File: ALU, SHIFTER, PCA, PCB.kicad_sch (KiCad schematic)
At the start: 14 parts

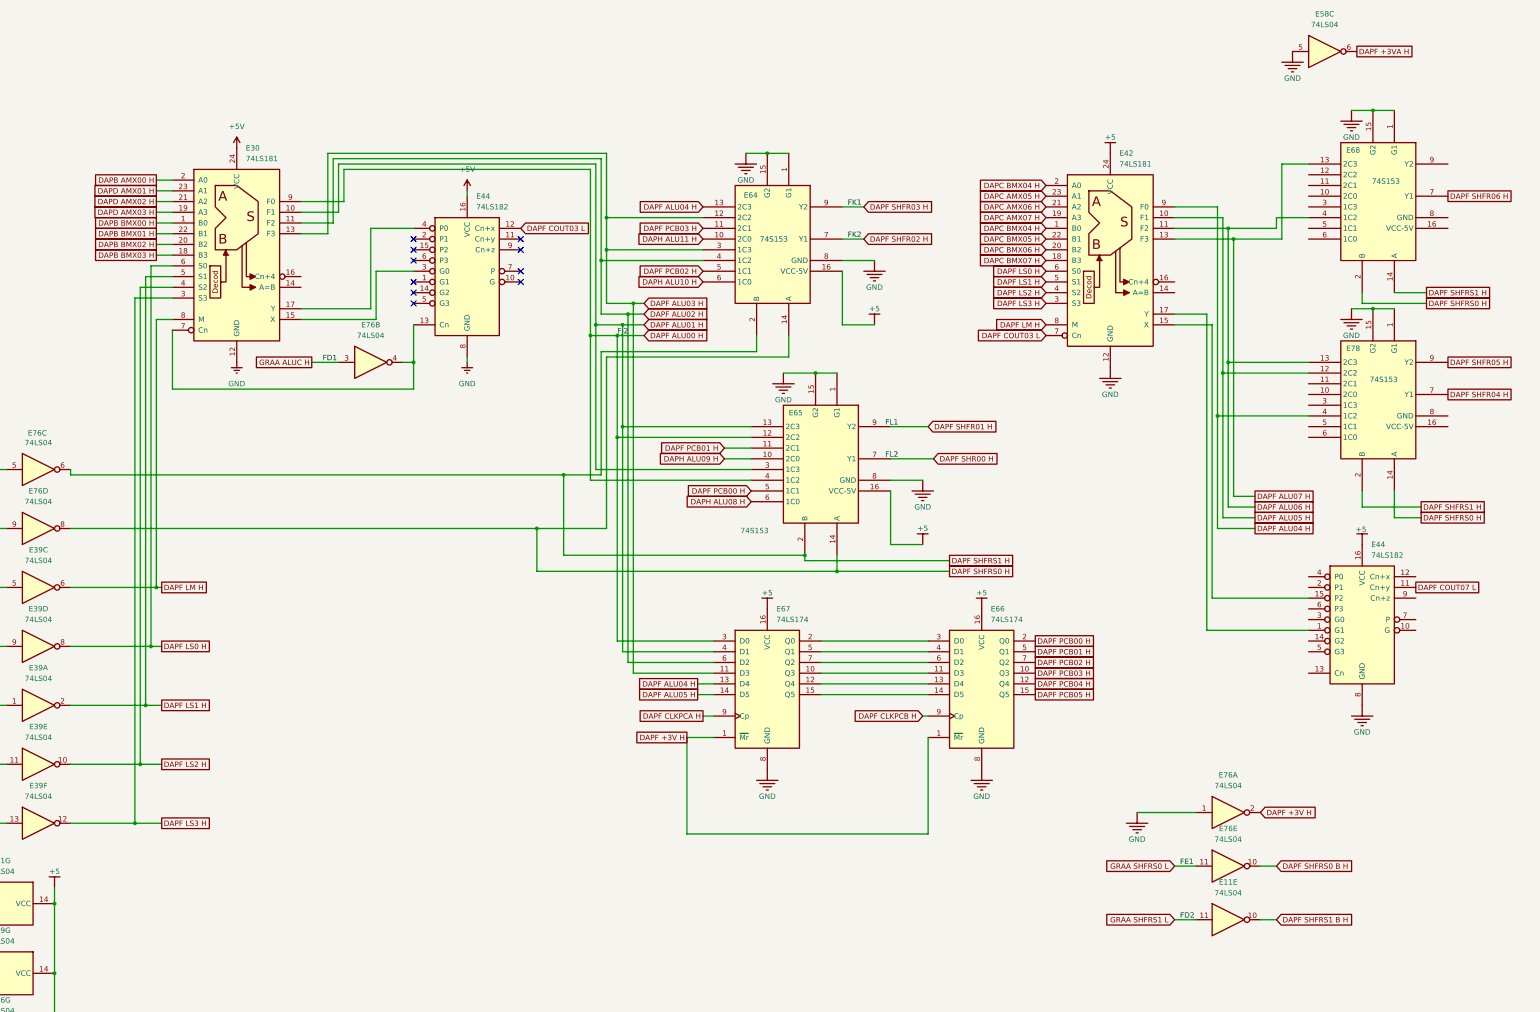
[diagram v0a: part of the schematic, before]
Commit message: updating to newest versions of schematics
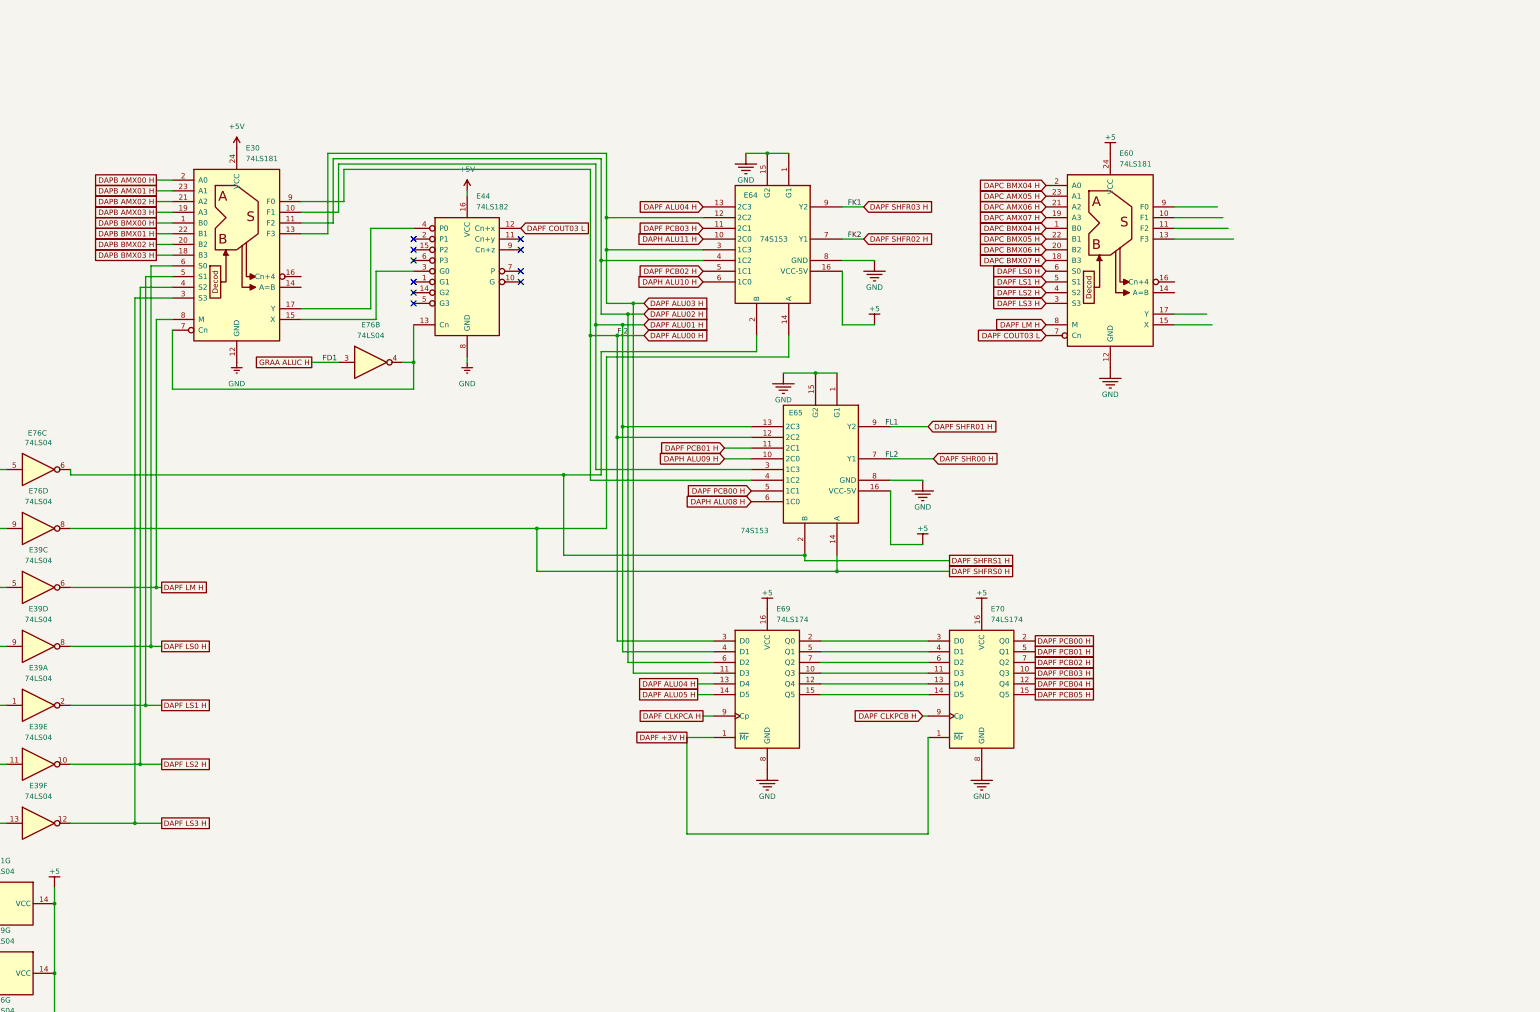
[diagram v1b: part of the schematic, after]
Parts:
- removed unit 5 of E11
- removed E44: 74LS182, symbol 74xx:74LS182
- removed unit 3 of E58
- removed E68, E78: 74S153, DIP16, symbol Untitled-altium-import:root_0_74S153
- removed unit 5 of E76
- removed unit 1 of E76
- renumbered E42 to E60, E67 to E69, E66 to E70
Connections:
- net DAPF ALU04 H: no longer E60.9 (F0)
- net DAPF ALU05 H: no longer E60.10 (F1)
- net DAPD AMX01 H renamed DAPB AMX01 H
- net DAPD AMX02 H renamed DAPB AMX02 H
- net DAPD AMX03 H renamed DAPB AMX03 H
- net DAPF ALU06 H: no longer names the net of E60.11 (F2)
- net DAPF ALU07 H: no longer names the net of E60.13 (F3)
